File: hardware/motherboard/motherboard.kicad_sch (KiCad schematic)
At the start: 82 parts, among them J1 IMU Connector, J2 JST-VH, J3 JST-VH, J4 JST-PH, J5 USB C 2.0, Q1 TSM7P06CP_ROG, Q2 TSM7P06CP_ROG, SW1 A, SW10 Right, SW11 Left, SW12 Up, SW13 Reset, SW2 B, SW3 X, SW4 Y, SW5 LB, SW6 RB, SW7 Start, SW8 Select, SW9 Down, U1 ESP32-S3-WROOM-1, U2 MCP73831-2-OT, U3 TPS75533KTTRG3, U4 TLV75709PDBV, U5 COM-09032

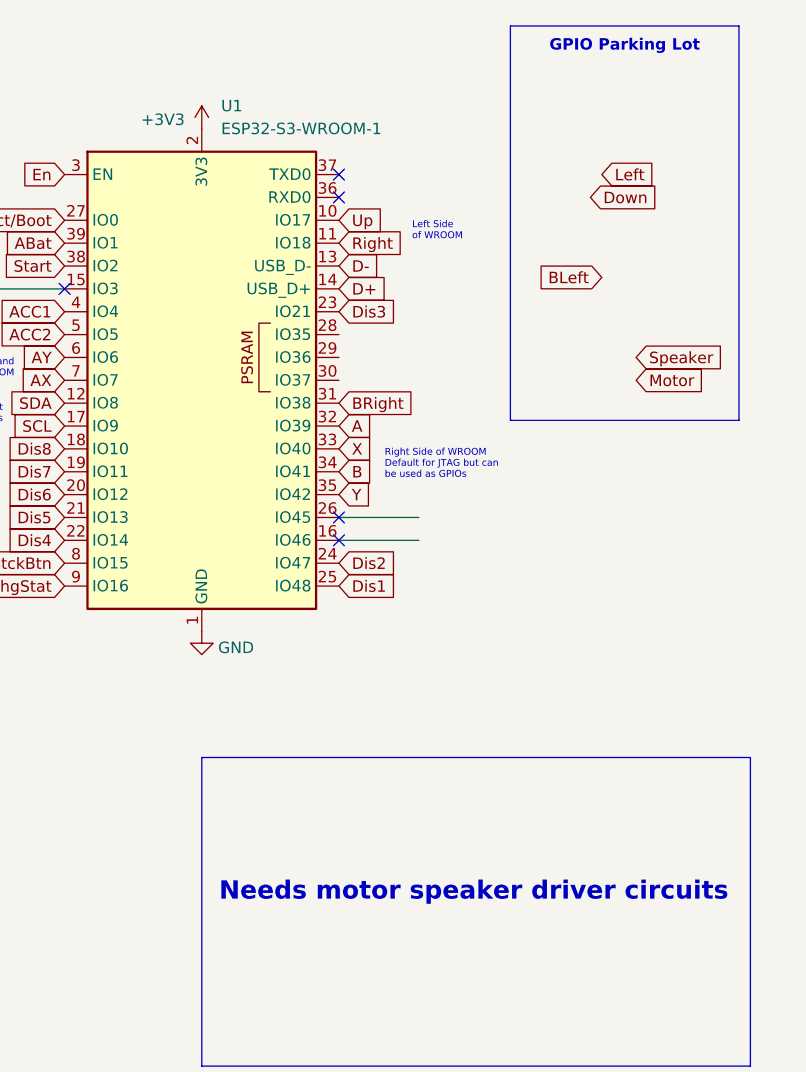
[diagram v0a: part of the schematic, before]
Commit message: Updated gpios
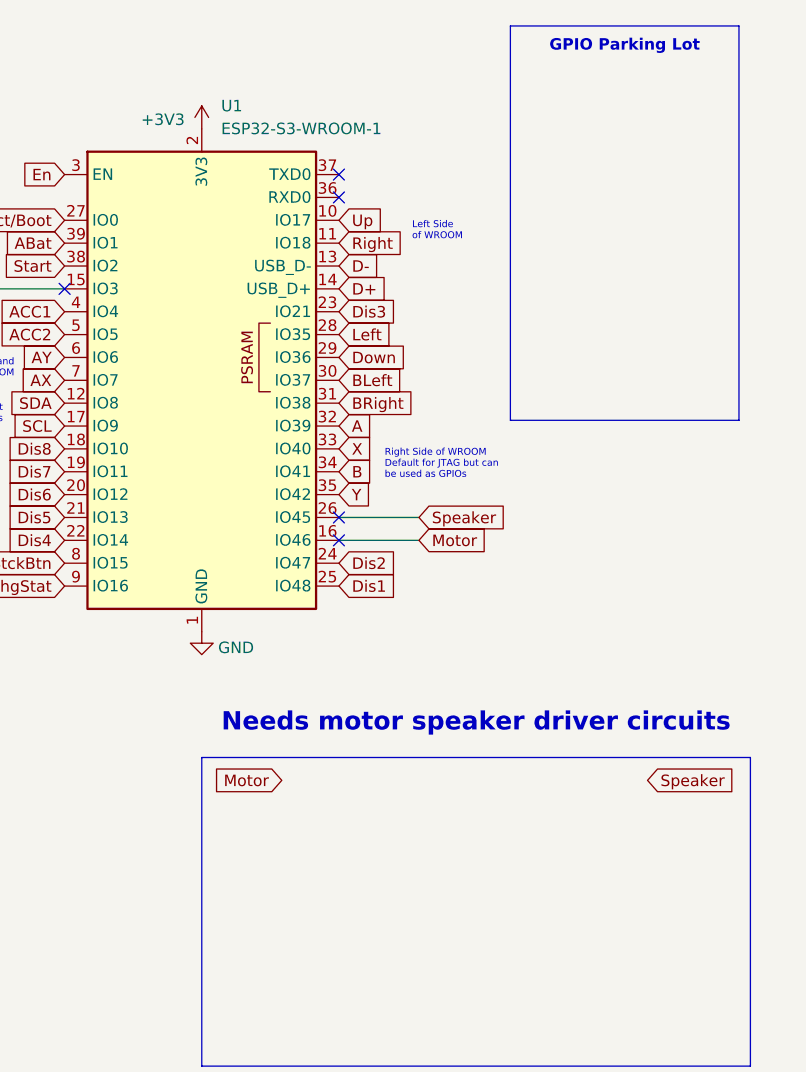
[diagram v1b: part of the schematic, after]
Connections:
- net BLeft: now also U1.30 (IO37)
- net Down: now also U1.29 (IO36)
- net Left: now also U1.28 (IO35)
- net Motor: now also U1.16 (IO46)
- net Speaker: now also U1.26 (IO45)
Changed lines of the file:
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@@
 	(text "Needs motor speaker driver circuits"
 		(exclude_from_sim no)
-		(at 252.476 110.236 0)
+		(at 252.73 91.44 0)
 		(effects
 			(font
@@
 	(global_label "BLeft"
 		(shape input)
-		(at 266.7 41.91 180)
+		(at 237.49 53.34 0)
 		(fields_autoplaced yes)
 		(effects
@@
 				(size 1.27 1.27)
 			)
-			(justify right)
+			(justify left)
 		)
 		(property "Intersheetrefs" "${INTERSHEET_REFS}"
-			(at 258.8767 41.91 0)
+			(at 245.3133 53.34 0)
 			(effects
 				(font
 					(size 1.27 1.27)
 				)
-				(justify right)
+				(justify left)
 				(hide yes)
 			)
@@
 	(global_label "Left"
 		(shape input)
-		(at 266.7 30.48 0)
+		(at 237.49 48.26 0)
 		(fields_autoplaced yes)
 		(effects
@@
 		)
 		(property "Intersheetrefs" "${INTERSHEET_REFS}"
-			(at 273.2533 30.48 0)
+			(at 244.0433 48.26 0)
 			(effects
 				(font
@@
 	(global_label "Speaker"
 		(shape input)
-		(at 270.51 50.8 0)
+		(at 246.38 68.58 0)
 		(fields_autoplaced yes)
 		(effects
@@
 		)
 		(property "Intersheetrefs" "${INTERSHEET_REFS}"
-			(at 280.9942 50.8 0)
+			(at 256.8642 68.58 0)
 			(effects
 				(font
@@
 		)
 	)
+	(global_label "Motor"
+		(shape input)
+		(at 231.14 97.79 180)
+		(fields_autoplaced yes)
+		(effects
+			(font
+				(size 1.27 1.27)
+			)
+			(justify right)
+		)
+		(property "Intersheetrefs" "${INTERSHEET_REFS}"
+			(at 222.8935 97.79 0)
+			(effects
+				(font
+					(size 1.27 1.27)
+				)
+				(justify right)
+				(hide yes)
+			)
+		)
+	)
 	(global_label "Select{slash}Boot"
 		(shape input)
@@
 	(global_label "Down"
 		(shape input)
-		(at 265.43 33.02 0)
+		(at 237.49 50.8 0)
 		(fields_autoplaced yes)
 		(effects
@@
 		)
 		(property "Intersheetrefs" "${INTERSHEET_REFS}"
-			(at 273.3137 33.02 0)
+			(at 245.3737 50.8 0)
 			(effects
 				(font
@@
 	(global_label "Motor"
 		(shape input)
-		(at 270.51 53.34 0)
+		(at 246.38 71.12 0)
+		(fields_autoplaced yes)
+		(effects
+			(font
+				(size 1.27 1.27)
+			)
+			(justify left)
+		)
+		(property "Intersheetrefs" "${INTERSHEET_REFS}"
+			(at 254.6265 71.12 0)
+			(effects
+				(font
+					(size 1.27 1.27)
+				)
+				(justify left)
+				(hide yes)
+			)
+		)
+	)
+	(global_label "Speaker"
+		(shape input)
+		(at 271.78 97.79 0)
 		(fields_autoplaced yes)
 		(effects
@@
 		)
 		(property "Intersheetrefs" "${INTERSHEET_REFS}"
-			(at 278.7565 53.34 0)
+			(at 282.2642 97.79 0)
 			(effects
 				(font
